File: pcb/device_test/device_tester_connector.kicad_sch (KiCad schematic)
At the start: 7 parts, among them J201 USB_C_Receptacle_USB2.0_16P, J202 Conn_01x04, J203 Conn_02x10_Row_Letter_First

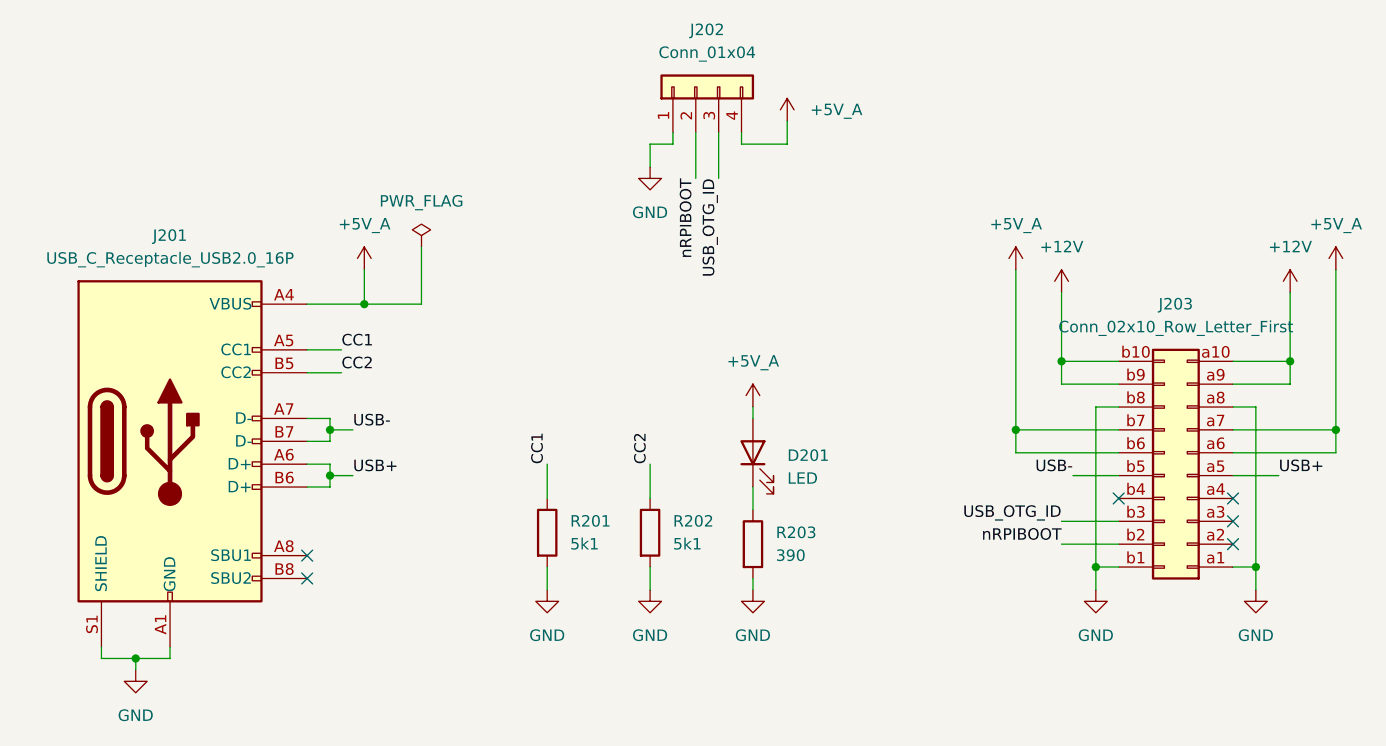
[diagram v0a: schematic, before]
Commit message: update
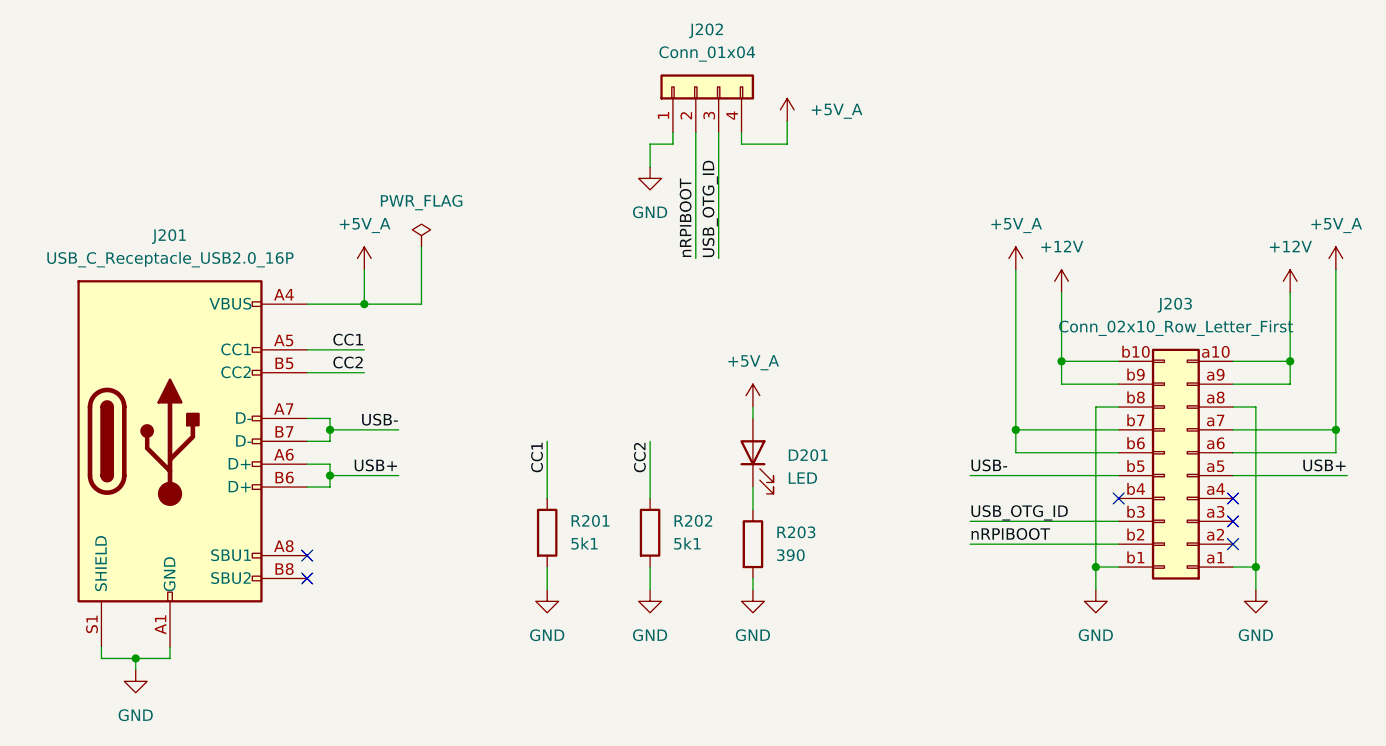
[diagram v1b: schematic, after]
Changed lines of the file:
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@@
 	(wire
 		(pts
-			(xy 144.78 63.5) (xy 144.78 68.58)
+			(xy 144.78 63.5) (xy 144.78 77.47)
 		)
 		(stroke
@@
 	(wire
 		(pts
-			(xy 104.14 101.6) (xy 106.68 101.6)
+			(xy 104.14 101.6) (xy 111.76 101.6)
 		)
 		(stroke
@@
 	(wire
 		(pts
-			(xy 186.69 101.6) (xy 191.77 101.6)
+			(xy 175.26 101.6) (xy 191.77 101.6)
 		)
 		(stroke
@@
 	(wire
 		(pts
-			(xy 101.6 87.63) (xy 105.41 87.63)
+			(xy 101.6 87.63) (xy 107.95 87.63)
 		)
 		(stroke
@@
 	(wire
 		(pts
-			(xy 204.47 101.6) (xy 209.55 101.6)
+			(xy 204.47 101.6) (xy 217.17 101.6)
 		)
 		(stroke
@@
 	(wire
 		(pts
-			(xy 104.14 96.52) (xy 106.68 96.52)
+			(xy 104.14 96.52) (xy 111.76 96.52)
 		)
 		(stroke
@@
 	(wire
 		(pts
-			(xy 139.7 100.33) (xy 139.7 104.14)
+			(xy 139.7 97.79) (xy 139.7 104.14)
 		)
 		(stroke
@@
 	(wire
 		(pts
-			(xy 101.6 90.17) (xy 105.41 90.17)
+			(xy 101.6 90.17) (xy 107.95 90.17)
 		)
 		(stroke
@@
 	(wire
 		(pts
-			(xy 185.42 109.22) (xy 191.77 109.22)
+			(xy 175.26 109.22) (xy 191.77 109.22)
 		)
 		(stroke
@@
 	(wire
 		(pts
-			(xy 185.42 106.68) (xy 191.77 106.68)
+			(xy 175.26 106.68) (xy 191.77 106.68)
 		)
 		(stroke
@@
 	(wire
 		(pts
-			(xy 147.32 63.5) (xy 147.32 68.58)
+			(xy 147.32 63.5) (xy 147.32 77.47)
 		)
 		(stroke
@@
 	(wire
 		(pts
-			(xy 128.27 100.33) (xy 128.27 104.14)
+			(xy 128.27 97.79) (xy 128.27 104.14)
 		)
 		(stroke
@@
 	)
 	(label "nRPIBOOT"
-		(at 185.42 109.22 180)
+		(at 175.26 109.22 0)
+		(effects
+			(font
+				(size 1.27 1.27)
+			)
+			(justify left bottom)
+		)
+	)
+	(label "USB-"
+		(at 111.76 96.52 180)
 		(effects
 			(font
@@
 		)
 	)
+	(label "nRPIBOOT"
+		(at 144.78 77.47 90)
+		(effects
+			(font
+				(size 1.27 1.27)
+			)
+			(justify left bottom)
+		)
+	)
+	(label "CC1"
+		(at 107.95 87.63 180)
+		(effects
+			(font
+				(size 1.27 1.27)
+			)
+			(justify right bottom)
+		)
+	)
+	(label "CC2"
+		(at 139.7 97.79 270)
+		(effects
+			(font
+				(size 1.27 1.27)
+			)
+			(justify right bottom)
+		)
+	)
+	(label "CC1"
+		(at 128.27 97.79 270)
+		(effects
+			(font
+				(size 1.27 1.27)
+			)
+			(justify right bottom)
+		)
+	)
+	(label "USB+"
+		(at 111.76 101.6 180)
+		(effects
+			(font
+				(size 1.27 1.27)
+			)
+			(justify right bottom)
+		)
+	)
+	(label "CC2"
+		(at 107.95 90.17 180)
+		(effects
+			(font
+				(size 1.27 1.27)
+			)
+			(justify right bottom)
+		)
+	)
 	(label "USB-"
-		(at 106.68 96.52 0)
+		(at 175.26 101.6 0)
 		(effects
 			(font
@@
 		)
 	)
-	(label "nRPIBOOT"
-		(at 144.78 68.58 270)
+	(label "USB+"
+		(at 217.17 101.6 180)
 		(effects
 			(font
@@
 		)
 	)
-	(label "CC1"
-		(at 105.41 87.63 0)
+	(label "USB_OTG_ID"
+		(at 175.26 106.68 0)
 		(effects
 			(font
@@
 		)
 	)
-	(label "CC2"
-		(at 139.7 100.33 90)
+	(label "USB_OTG_ID"
+		(at 147.32 77.47 90)
 		(effects
 			(font
@@
 		)
 	)
-	(label "CC1"
-		(at 128.27 100.33 90)
-		(effects
-			(font
-				(size 1.27 1.27)
-			)
-			(justify left bottom)
-		)
-	)
-	(label "USB+"
-		(at 106.68 101.6 0)
-		(effects
-			(font
-				(size 1.27 1.27)
-			)
-			(justify left bottom)
-		)
-	)
-	(label "CC2"
-		(at 105.41 90.17 0)
-		(effects
-			(font
-				(size 1.27 1.27)
-			)
-			(justify left bottom)
-		)
-	)
-	(label "USB-"
-		(at 186.69 101.6 180)
-		(effects
-			(font
-				(size 1.27 1.27)
-			)
-			(justify right bottom)
-		)
-	)
-	(label "USB+"
-		(at 209.55 101.6 0)
-		(effects
-			(font
-				(size 1.27 1.27)
-			)
-			(justify left bottom)
-		)
-	)
-	(label "USB_OTG_ID"
-		(at 185.42 106.68 180)
-		(effects
-			(font
-				(size 1.27 1.27)
-			)
-			(justify right bottom)
-		)
-	)
-	(label "USB_OTG_ID"
-		(at 147.32 68.58 270)
-		(effects
-			(font
-				(size 1.27 1.27)
-			)
-			(justify right bottom)
-		)
-	)
